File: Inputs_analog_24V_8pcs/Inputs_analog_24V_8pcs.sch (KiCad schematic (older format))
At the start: 16 parts, among them J1 Screw_Terminal_01x02, J2 Screw_Terminal_01x02, J3 Screw_Terminal_01x06, U1 SN74HC14N, U2 SN74HC14N, U3 74HC151N.652

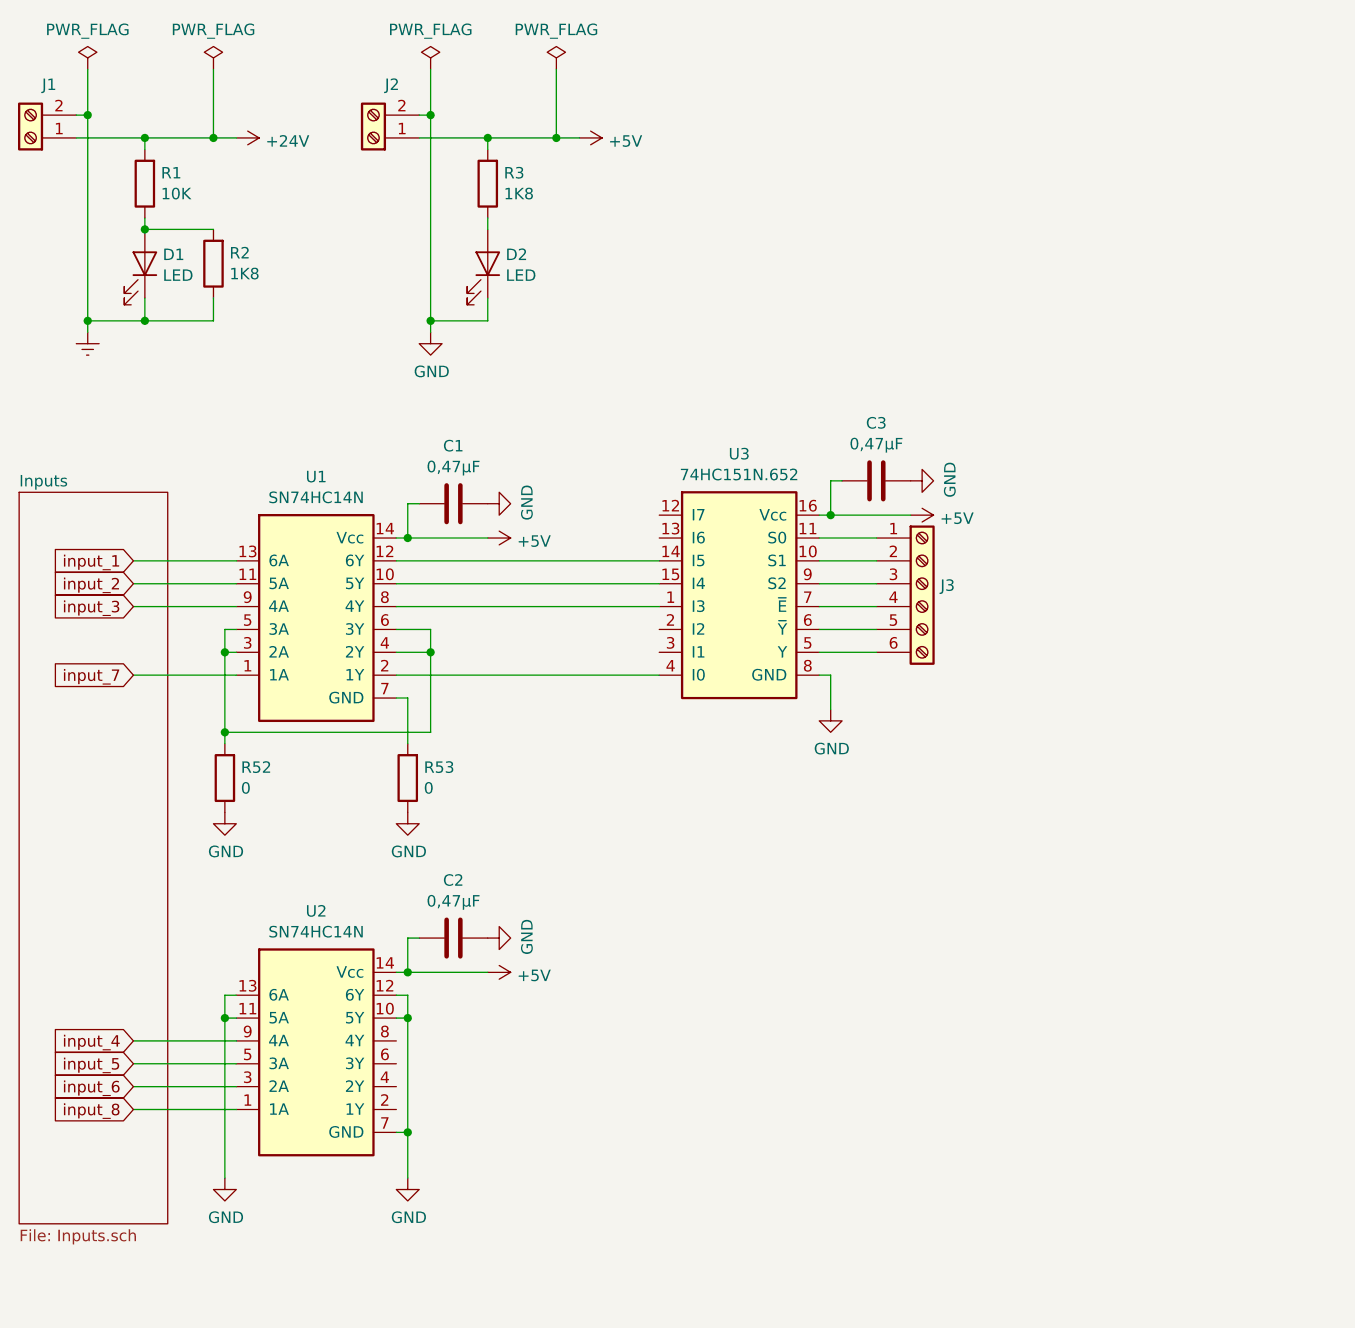
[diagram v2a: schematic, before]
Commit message: Finish pcb
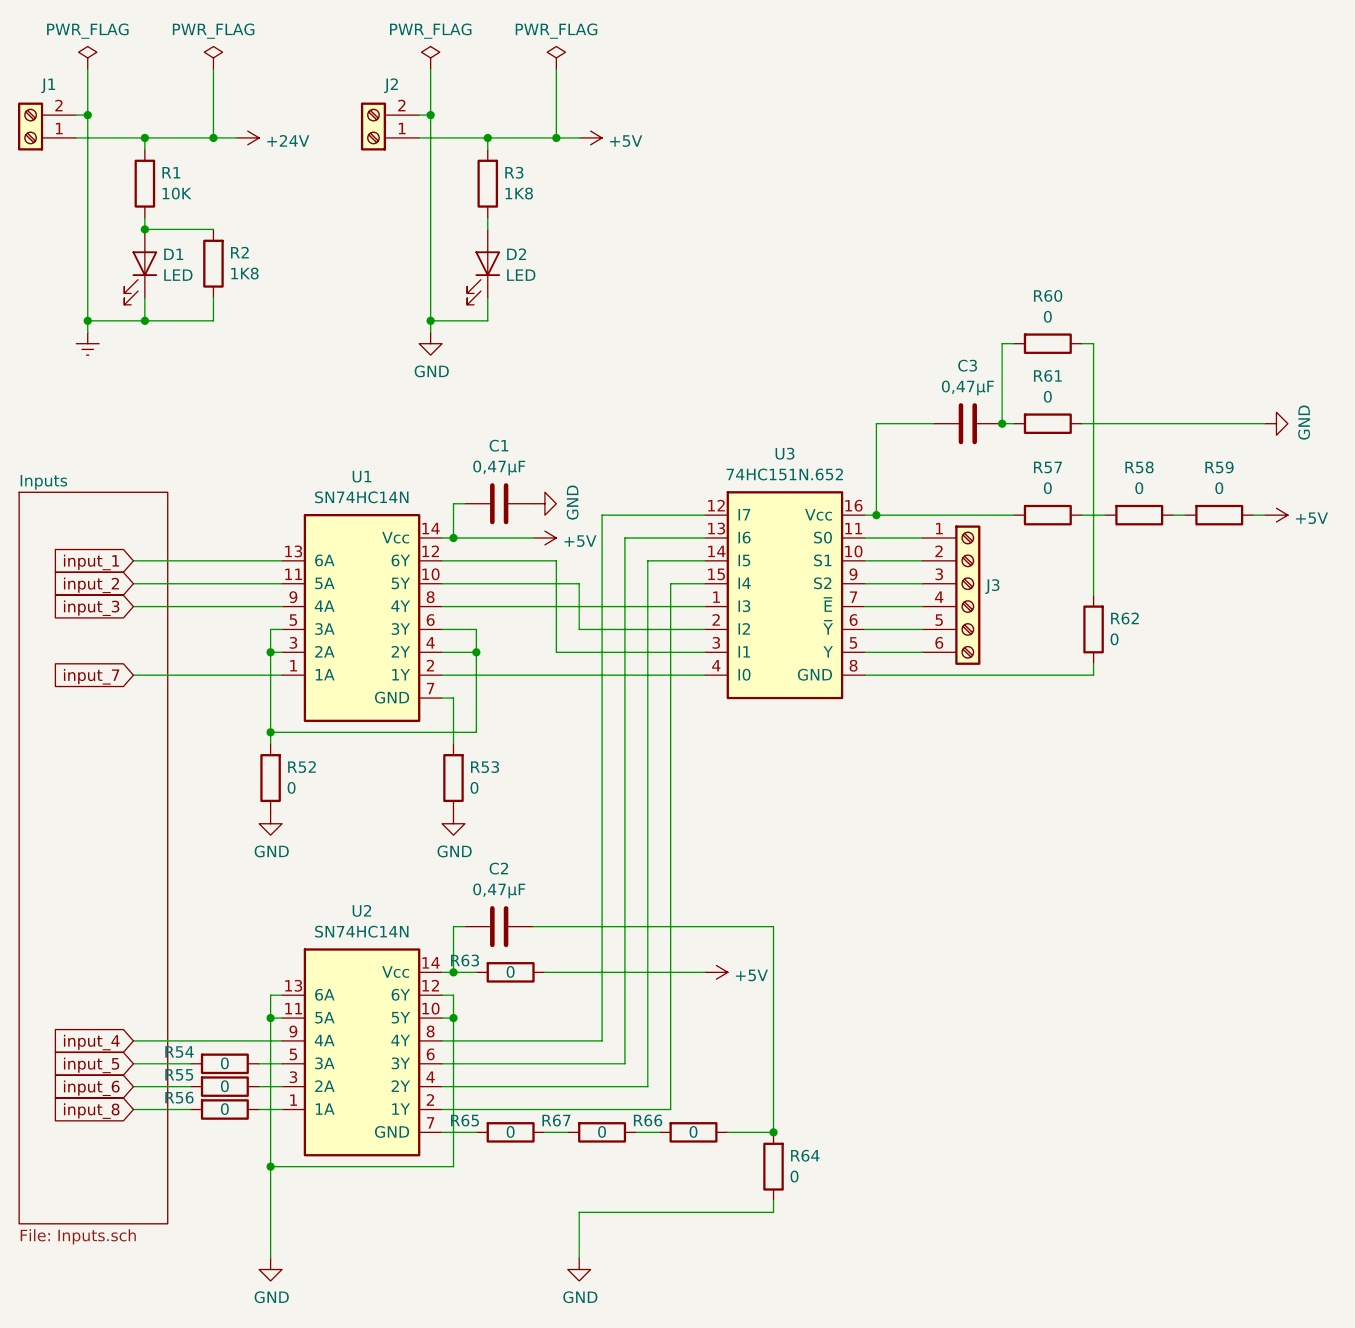
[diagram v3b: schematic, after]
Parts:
- added R54, R55, R56, R57, R58, R59, R60, R61, R62, R63, R64, R65, R66, R67: 0, Resistor_THT:R_Axial_DIN0207_L6.3mm_D2.5mm_P7.62mm_Horizontal, symbol Device:R
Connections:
- net +5V: now also R59.1, R63.1; no longer C2.2, C3.2, U2.14 (Vcc), U3.16 (Vcc)
- net GND: now also R61.1, R64.1; no longer C2.1, C3.1, U2.7 (GND), U3.8 (GND)
- net input_5: now also R54.2; no longer U2.5 (3A)
- net input_6: now also R55.2; no longer U2.3 (2A)
- net input_8: now also R56.2; no longer U2.1 (1A)
- net at U1.10 (5Y): now also U3.2 (I2); no longer U3.15 (I4)
- net at U1.12 (6Y): now also U3.3 (I1); no longer U3.14 (I5)
- net at U2.2 (1Y): now also U3.15 (I4)
- net at U2.4 (2Y): now also U3.14 (I5)
- net at U2.6 (3Y): now also U3.13 (I6)
- net at U2.8 (4Y): now also U3.12 (I7)
- new net: R54.1, U2.5 (3A)
- new net: R55.1, U2.3 (2A)
- new net: R56.1, U2.1 (1A)
- new net: R57.1, R58.2
- new net: C3.2, R57.2, U3.16 (Vcc)
- new net: R58.1, R59.2
- new net: R60.1, R62.2
- new net: C3.1, R60.2, R61.2
- new net: R62.1, U3.8 (GND)
- new net: C2.2, R63.2, U2.14 (Vcc)
- new net: C2.1, R64.2, R66.1
- new net: R66.2, R67.1
- new net: R65.1, R67.2
- new net: R65.2, U2.7 (GND)
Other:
- moved on the sheet: C1, C2, C3, J3, R52, R53, U1, U2, U3
